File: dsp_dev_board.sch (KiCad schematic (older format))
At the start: 23 parts, among them J1 9v_jack, J2 aux_mcu_power, J3 input_jack, J7 output_jack, J8 audio_in, J9 audio_out, U1 TL072, U101 TL072, U102 AMS1117-3.3

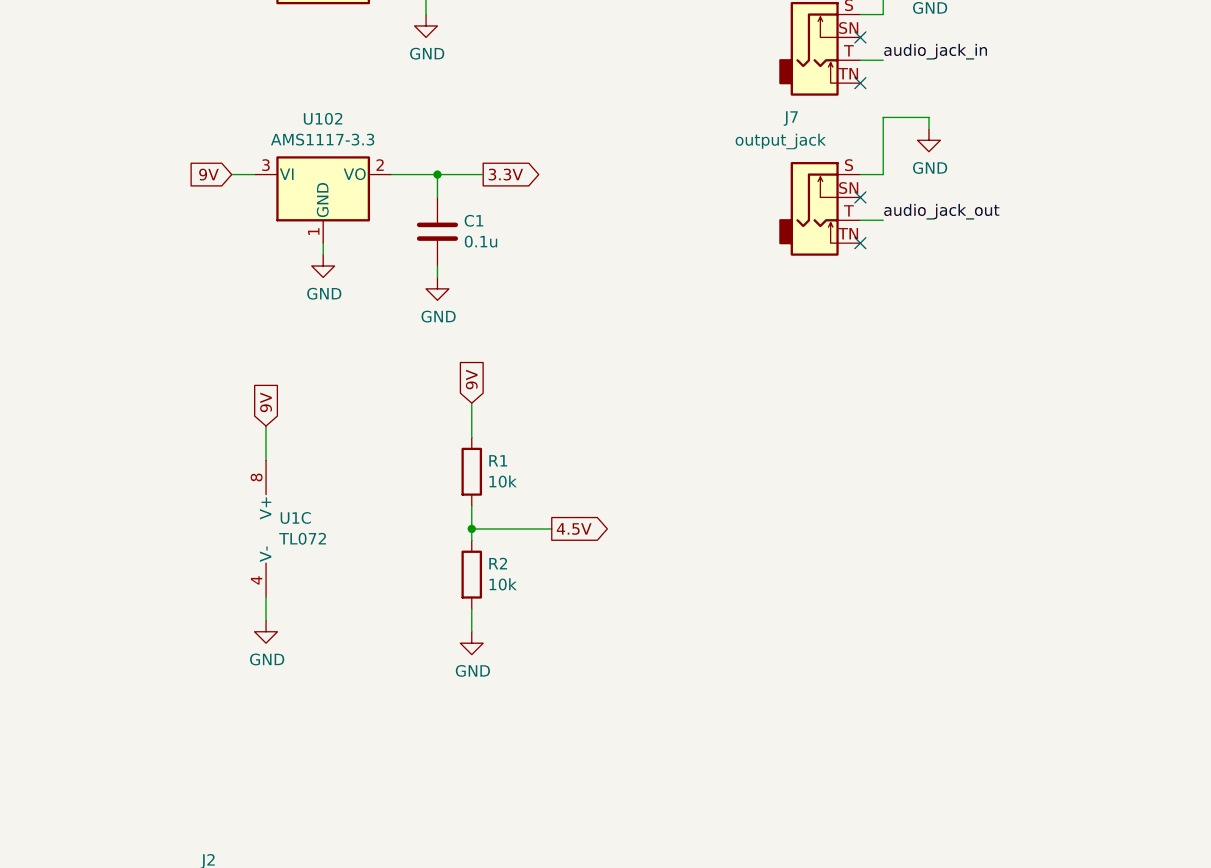
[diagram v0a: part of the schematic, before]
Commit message: USB
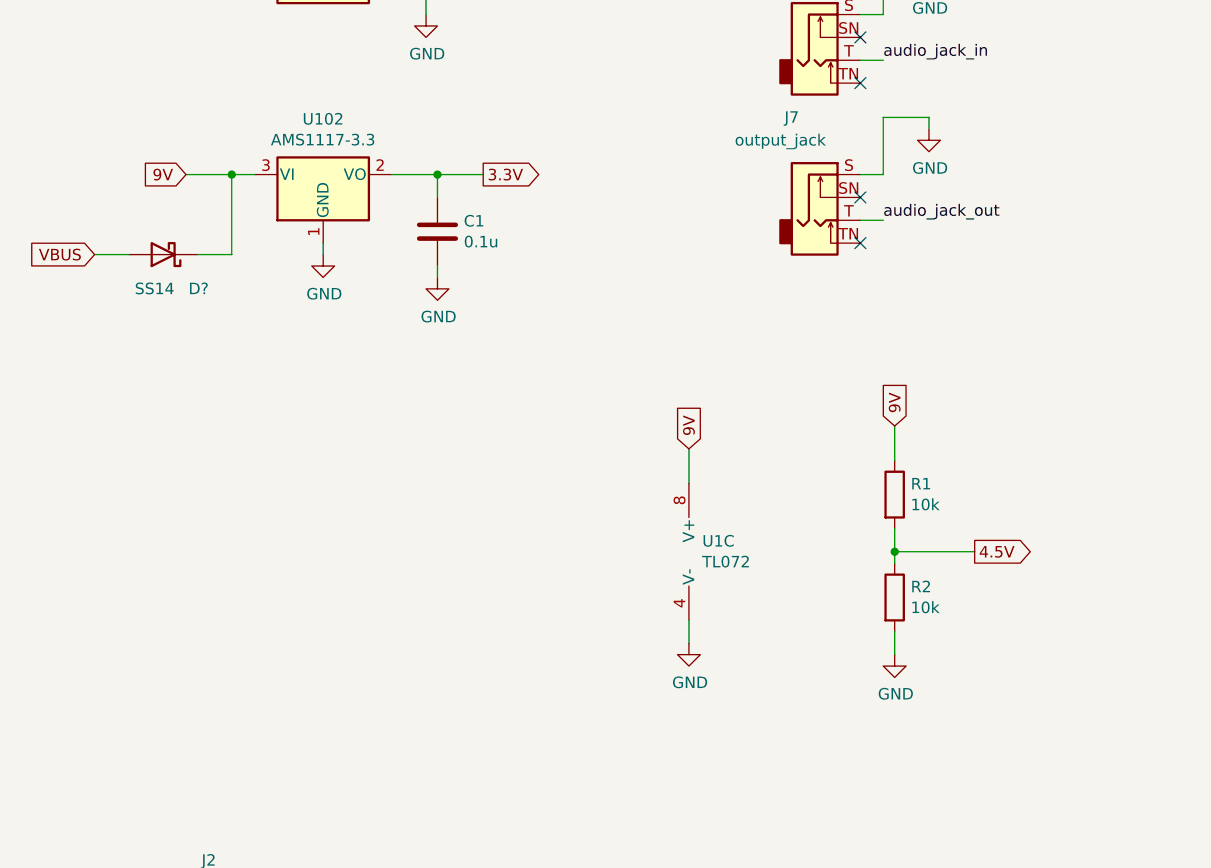
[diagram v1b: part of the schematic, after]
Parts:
- added D?: SS14, symbol Device:D_Schottky
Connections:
- net 9V: now also D?.1 (K)
- new net VBUS: D?.2 (A)
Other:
- moved on the sheet: R1, R2, U1C
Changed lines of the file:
@@
 Wire Wire Line
 	6850 1900 7050 1900
-Text GLabel 2700 3400 1    50   Input ~ 0
+Text GLabel 4550 3500 1    50   Input ~ 0
 9V
 $Comp
 L Device:R R1
 U 1 1 600A09B1
-P 2700 3700
-F 0 "R1" H 2770 3746 50  0000 L CNN
-F 1 "10k" H 2770 3655 50  0000 L CNN
-F 2 "" V 2630 3700 50  0001 C CNN
-F 3 "~" H 2700 3700 50  0001 C CNN
-	1    2700 3700
+P 4550 3800
+F 0 "R1" H 4620 3846 50  0000 L CNN
+F 1 "10k" H 4620 3755 50  0000 L CNN
+F 2 "" V 4480 3800 50  0001 C CNN
+F 3 "~" H 4550 3800 50  0001 C CNN
+	1    4550 3800
 	1    0    0    -1
 $EndComp
@@
 L Device:R R2
 U 1 1 600A106D
-P 2700 4150
-F 0 "R2" H 2770 4196 50  0000 L CNN
-F 1 "10k" H 2770 4105 50  0000 L CNN
-F 2 "" V 2630 4150 50  0001 C CNN
-F 3 "~" H 2700 4150 50  0001 C CNN
-	1    2700 4150
-	1    0    0    -1
-$EndComp
-Wire Wire Line
-	2700 3850 2700 3950
+P 4550 4250
+F 0 "R2" H 4620 4296 50  0000 L CNN
+F 1 "10k" H 4620 4205 50  0000 L CNN
+F 2 "" V 4480 4250 50  0001 C CNN
+F 3 "~" H 4550 4250 50  0001 C CNN
+	1    4550 4250
+	1    0    0    -1
+$EndComp
+Wire Wire Line
+	4550 3950 4550 4050
 $Comp
 L power:GND #PWR02
 U 1 1 600A2818
-P 2700 4400
-F 0 "#PWR02" H 2700 4150 50  0001 C CNN
-F 1 "GND" H 2705 4227 50  0000 C CNN
-F 2 "" H 2700 4400 50  0001 C CNN
-F 3 "" H 2700 4400 50  0001 C CNN
-	1    2700 4400
-	1    0    0    -1
-$EndComp
-Wire Wire Line
-	2700 4400 2700 4300
-Wire Wire Line
-	2700 3400 2700 3550
-Wire Wire Line
-	2700 3950 3050 3950
-Connection ~ 2700 3950
-Wire Wire Line
-	2700 3950 2700 4000
-Text GLabel 3050 3950 2    50   Output ~ 0
+P 4550 4500
+F 0 "#PWR02" H 4550 4250 50  0001 C CNN
+F 1 "GND" H 4555 4327 50  0000 C CNN
+F 2 "" H 4550 4500 50  0001 C CNN
+F 3 "" H 4550 4500 50  0001 C CNN
+	1    4550 4500
+	1    0    0    -1
+$EndComp
+Wire Wire Line
+	4550 4500 4550 4400
+Wire Wire Line
+	4550 3500 4550 3650
+Wire Wire Line
+	4550 4050 4900 4050
+Connection ~ 4550 4050
+Wire Wire Line
+	4550 4050 4550 4100
+Text GLabel 4900 4050 2    50   Output ~ 0
 4.5V
 Text GLabel 7950 1700 0    50   Input ~ 0
@@
 L Amplifier_Operational:TL072 U1
 U 3 1 600C8CB7
-P 1900 3950
-F 0 "U1" H 1858 3996 50  0000 L CNN
-F 1 "TL072" H 1858 3905 50  0000 L CNN
-F 2 "" H 1900 3950 50  0001 C CNN
-F 3 "http://www.ti.com/lit/ds/symlink/tl071.pdf" H 1900 3950 50  0001 C CNN
-	3    1900 3950
-	1    0    0    -1
-$EndComp
-Text GLabel 1800 3500 1    50   Input ~ 0
+P 3750 4050
+F 0 "U1" H 3708 4096 50  0000 L CNN
+F 1 "TL072" H 3708 4005 50  0000 L CNN
+F 2 "" H 3750 4050 50  0001 C CNN
+F 3 "http://www.ti.com/lit/ds/symlink/tl071.pdf" H 3750 4050 50  0001 C CNN
+	3    3750 4050
+	1    0    0    -1
+$EndComp
+Text GLabel 3650 3600 1    50   Input ~ 0
 9V
 Wire Wire Line
-	1800 3500 1800 3650
+	3650 3600 3650 3750
 $Comp
 L power:GND #PWR01
 U 1 1 600D21C7
-P 1800 4350
-F 0 "#PWR01" H 1800 4100 50  0001 C CNN
-F 1 "GND" H 1805 4177 50  0000 C CNN
-F 2 "" H 1800 4350 50  0001 C CNN
-F 3 "" H 1800 4350 50  0001 C CNN
-	1    1800 4350
-	1    0    0    -1
-$EndComp
-Wire Wire Line
-	1800 4350 1800 4250
+P 3650 4450
+F 0 "#PWR01" H 3650 4200 50  0001 C CNN
+F 1 "GND" H 3655 4277 50  0000 C CNN
+F 2 "" H 3650 4450 50  0001 C CNN
+F 3 "" H 3650 4450 50  0001 C CNN
+	1    3650 4450
+	1    0    0    -1
+$EndComp
+Wire Wire Line
+	3650 4450 3650 4350
 Wire Wire Line
 	6900 5150 7550 5150
@@
 Wire Wire Line
 	1750 2400 1650 2400
-Text GLabel 1650 2400 0    50   Input ~ 0
+Text GLabel 1450 2400 0    50   Input ~ 0
 9V
 Wire Wire Line
@@
 Wire Wire Line
 	2150 6950 2000 6950
+$Comp
+L Device:D_Schottky D?
+U 1 1 6020CE2E
+P 1350 2750
+F 0 "D?" H 1150 2900 50  0000 L CNN
+F 1 "SS14" H 1300 2900 50  0000 L CNN
+F 2 "" H 1350 2750 50  0001 C CNN
+F 3 "~" H 1350 2750 50  0001 C CNN
+	1    1350 2750
+	-1   0    0    1
+$EndComp
+Text GLabel 1050 2750 0    50   Input ~ 0
+VBUS
+Wire Wire Line
+	1500 2750 1650 2750
+Wire Wire Line
+	1650 2750 1650 2400
+Connection ~ 1650 2400
+Wire Wire Line
+	1650 2400 1450 2400
+Wire Wire Line
+	1200 2750 1050 2750
 $EndSCHEMATC
